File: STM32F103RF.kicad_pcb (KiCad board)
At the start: 4 copper layers, 68 x 24 mm, 56 parts, among them J1 USB_C_Receptacle_USB2.0, J2 Conn_01x04, J3 Conn_Coaxial, U1 SPX3819M5-L-3-3, U2 STM32F103C6Tx, U3 NRF24L01, Y1 16MHz, Y2 16MHz

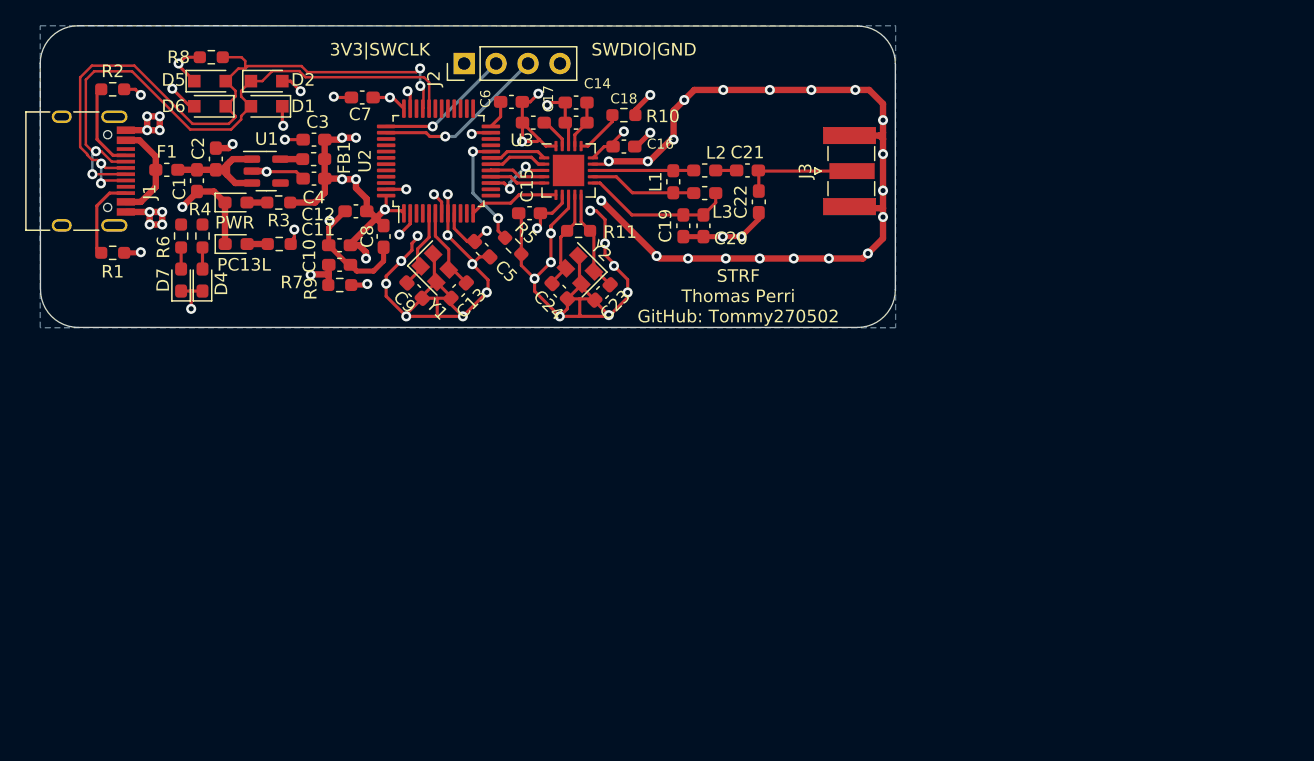
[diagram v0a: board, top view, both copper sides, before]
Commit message: added pictures and BOM
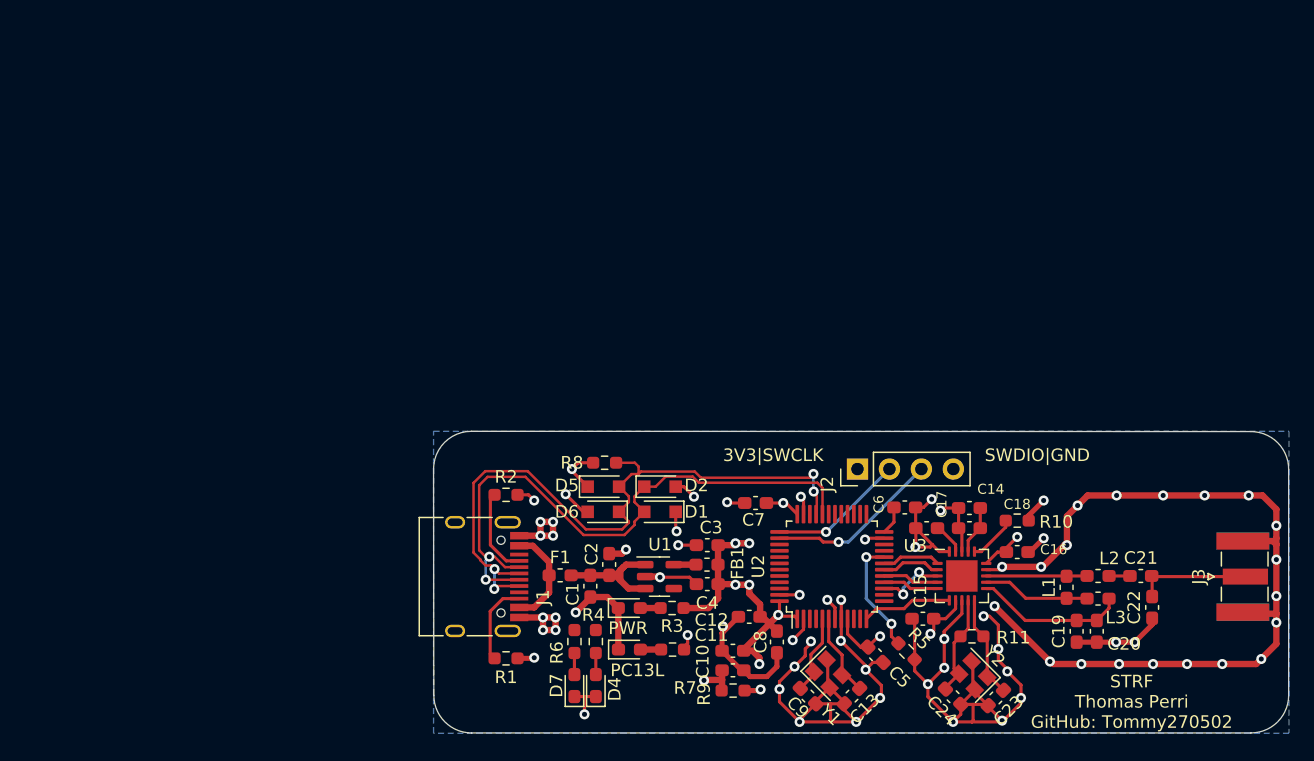
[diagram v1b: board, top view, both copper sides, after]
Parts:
- moved C2 44.9 mm to (81.2, 61.8)
- moved C20 44.9 mm to (120.0, 67.1)
- moved D4 44.9 mm to (80.2, 71.5)
- moved R4 44.9 mm to (80.2, 68.0)
- moved C11 44.9 mm to (91.1, 68.7)
- moved C14 44.9 mm to (109.9, 57.3)
- moved C15 44.9 mm to (106.2, 66.1)
- moved C18 44.9 mm to (109.9, 58.9)
- moved C19 44.9 mm to (118.4, 67.1)
- moved C21 44.9 mm to (123.5, 62.7)
- moved C24 44.9 mm to (108.6, 72.3)
- moved C4 44.9 mm to (89.0, 63.4)
- moved C5 44.9 mm to (102.4, 69.0)
- moved D1 44.9 mm to (85.3, 57.6)
- moved D2 44.9 mm to (85.3, 55.6)
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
